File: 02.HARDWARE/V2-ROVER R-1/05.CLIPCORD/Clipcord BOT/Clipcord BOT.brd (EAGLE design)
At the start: 21.7 x 13.1 mm, 3 parts

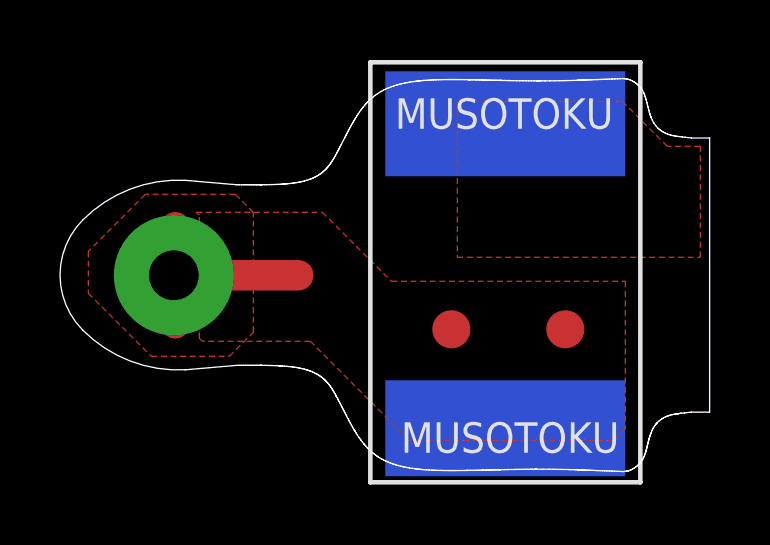
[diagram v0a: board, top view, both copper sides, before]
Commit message: Cambios menores antes de pedido
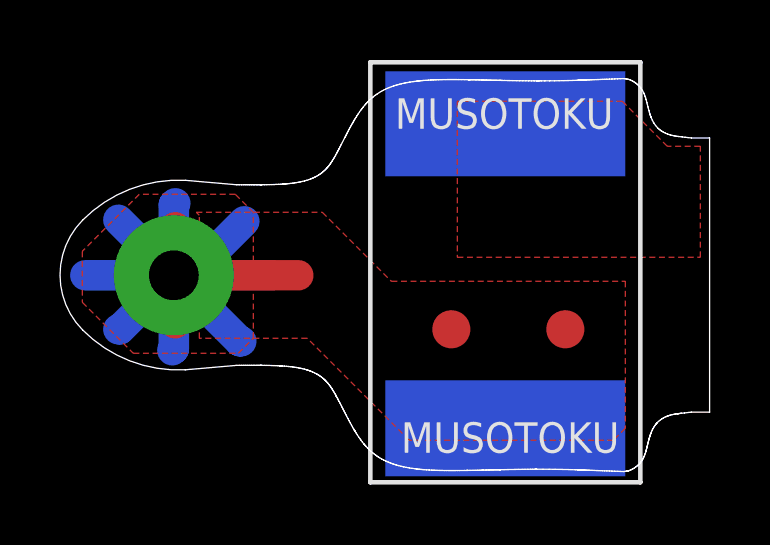
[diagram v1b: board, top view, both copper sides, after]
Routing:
- net LINE: track 7.39 -> 32.4 mm
- added copper zone on layer 16, net N$2
